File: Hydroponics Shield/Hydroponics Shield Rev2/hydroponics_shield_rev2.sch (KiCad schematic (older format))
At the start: 85 parts, among them CON1 PJ-202A, J1 282836-6, J2 282836-6, J3 RJHSE-5080, P2 0022053031, P3 MTG, P4 22-05-3021, P5 22-05-3021, P6 MTG, P7 MTG, P8 MTG, P9 0731000105, Q1 DMN65D8L-7, Q5 PSMN022-30PL,127, Q6 PSMN022-30PL,127, Q7 PSMN022-30PL,127, Q8 PSMN022-30PL,127, Q9 PSMN022-30PL,127, U1 LMC6482IN, U2 PCF8563, U3 AZ1117CH-3_3TRG1, Y1 CFS-20632768DZFB

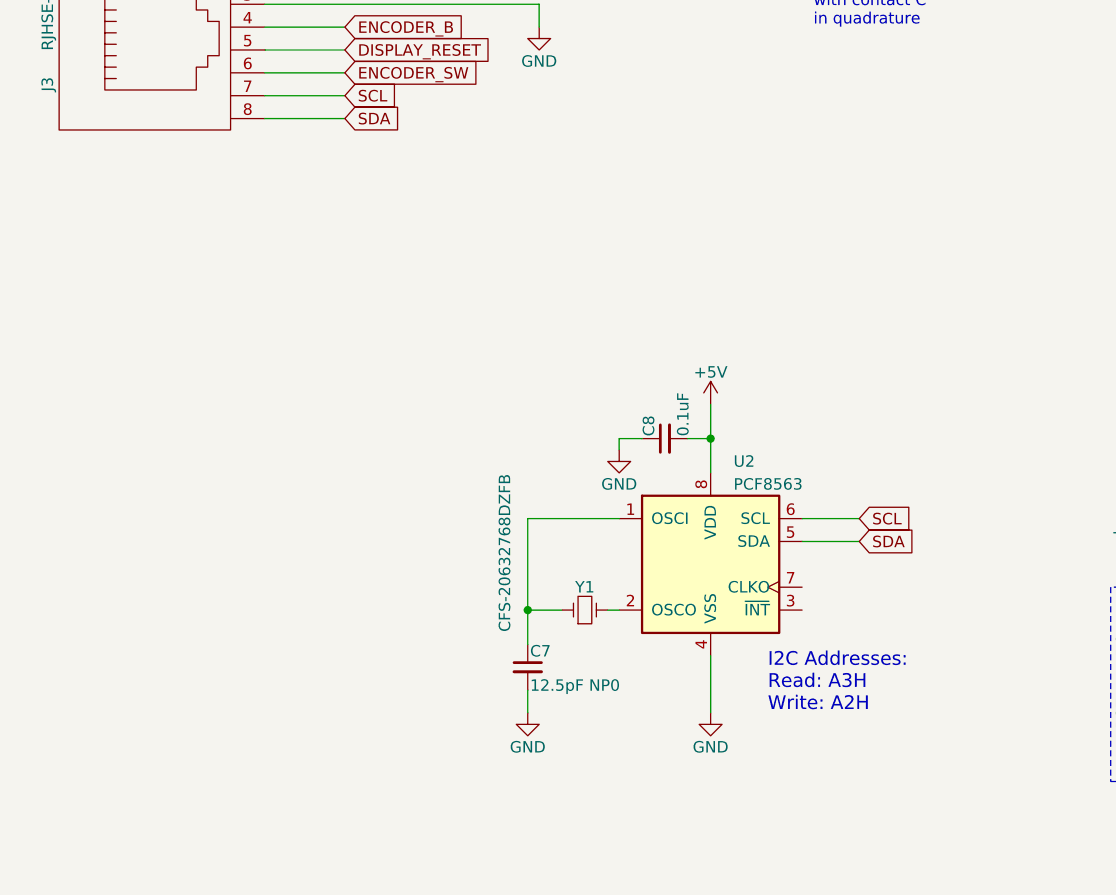
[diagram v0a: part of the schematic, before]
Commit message: .
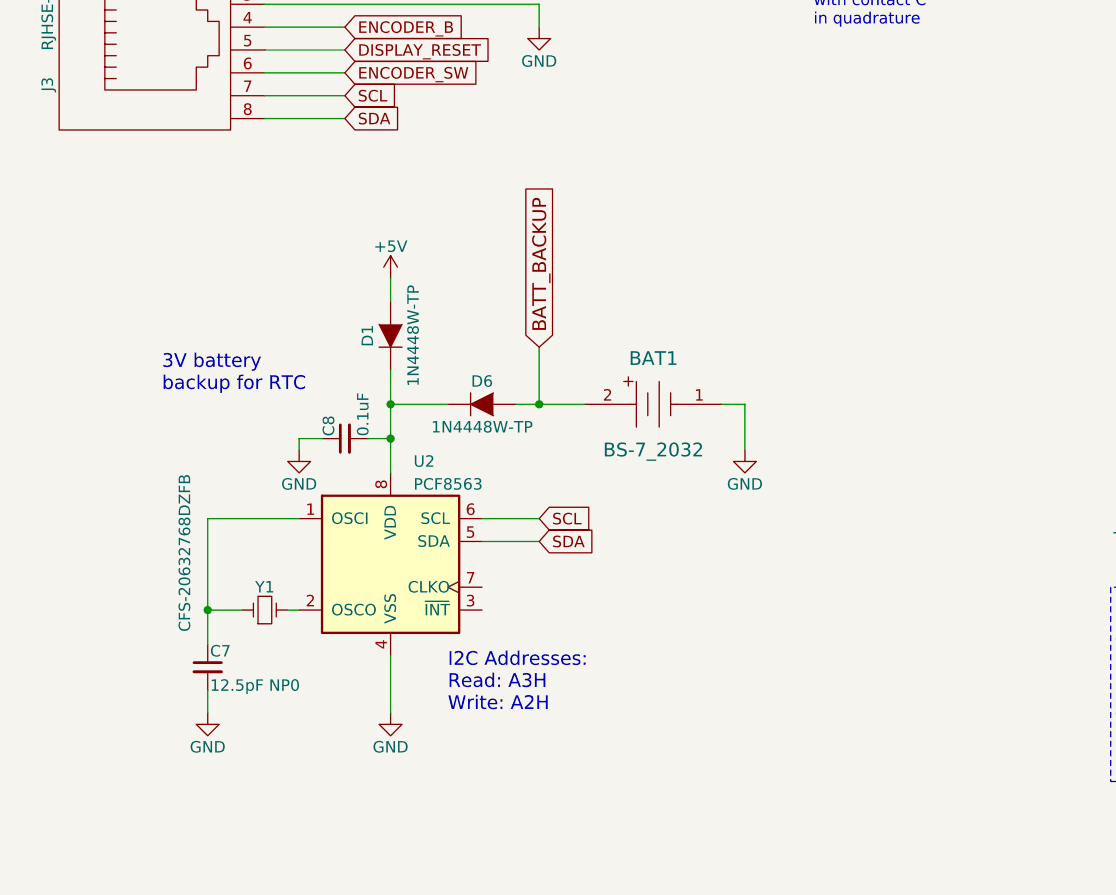
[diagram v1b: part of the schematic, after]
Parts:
- added BAT1: BS-7_2032, USER_CONNECTORS:BS-7_USER, symbol BS-7_2032
- added D1, D6: 1N4448W-TP, Diodes_SMD:SOD-123, symbol 1N4448W-TP
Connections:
- net +5V: now also D1.2 (A); no longer C8.2, U2.8 (VDD)
- net GND: now also BAT1.1
- new net: C8.2, D1.1 (K), D6.1 (K), U2.8 (VDD)
- new net BATT_BACKUP: BAT1.2, D6.2 (A)
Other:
- note added: "3V battery \nbackup for RTC"
- moved on the sheet: C7, C8, U2, Y1
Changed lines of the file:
@@
 L PCF8563 U2
 U 1 1 5B08C32E
-P 3750 9100
-F 0 "U2" H 3850 9550 50  0000 L CNN
-F 1 "PCF8563" H 3850 9450 50  0000 L CNN
-F 2 "digikey-footprints:8-SOIC" H 3750 9100 50  0001 C CNN
-F 3 "" H 3750 9100 50  0000 C CNN
-	1    3750 9100
-	1    0    0    -1
-$EndComp
-Wire Wire Line
-	3350 8900 2950 8900
-Wire Wire Line
-	2950 8900 2950 9450
-Wire Wire Line
-	2950 9300 3100 9300
-Wire Wire Line
-	3300 9300 3350 9300
-Connection ~ 2950 9300
+P 2350 9100
+F 0 "U2" H 2450 9550 50  0000 L CNN
+F 1 "PCF8563" H 2450 9450 50  0000 L CNN
+F 2 "digikey-footprints:8-SOIC" H 2350 9100 50  0001 C CNN
+F 3 "" H 2350 9100 50  0000 C CNN
+	1    2350 9100
+	1    0    0    -1
+$EndComp
+Wire Wire Line
+	1950 8900 1550 8900
+Wire Wire Line
+	1550 8900 1550 9450
+Wire Wire Line
+	1550 9300 1700 9300
+Wire Wire Line
+	1900 9300 1950 9300
+Connection ~ 1550 9300
 $Comp
 L C_Small C7
 U 1 1 5B091E53
-P 2950 9550
-F 0 "C7" H 2960 9620 50  0000 L CNN
-F 1 "12.5pF NP0" H 2960 9470 50  0000 L CNN
-F 2 "Capacitors_SMD:C_0805_HandSoldering" H 2950 9550 50  0001 C CNN
-F 3 "" H 2950 9550 50  0000 C CNN
-	1    2950 9550
-	1    0    0    -1
-$EndComp
-Wire Wire Line
-	2950 9650 2950 9750
+P 1550 9550
+F 0 "C7" H 1560 9620 50  0000 L CNN
+F 1 "12.5pF NP0" H 1560 9470 50  0000 L CNN
+F 2 "Capacitors_SMD:C_0805_HandSoldering" H 1550 9550 50  0001 C CNN
+F 3 "" H 1550 9550 50  0000 C CNN
+	1    1550 9550
+	1    0    0    -1
+$EndComp
+Wire Wire Line
+	1550 9650 1550 9750
 $Comp
 L GND #PWR051
 U 1 1 5B09286D
-P 2950 9750
-F 0 "#PWR051" H 2950 9500 50  0001 C CNN
-F 1 "GND" H 2950 9600 50  0000 C CNN
-F 2 "" H 2950 9750 50  0000 C CNN
-F 3 "" H 2950 9750 50  0000 C CNN
-	1    2950 9750
+P 1550 9750
+F 0 "#PWR051" H 1550 9500 50  0001 C CNN
+F 1 "GND" H 1550 9600 50  0000 C CNN
+F 2 "" H 1550 9750 50  0000 C CNN
+F 3 "" H 1550 9750 50  0000 C CNN
+	1    1550 9750
 	1    0    0    -1
 $EndComp
@@
 L GND #PWR052
 U 1 1 5B093393
-P 3750 9750
-F 0 "#PWR052" H 3750 9500 50  0001 C CNN
-F 1 "GND" H 3750 9600 50  0000 C CNN
-F 2 "" H 3750 9750 50  0000 C CNN
-F 3 "" H 3750 9750 50  0000 C CNN
-	1    3750 9750
-	1    0    0    -1
-$EndComp
-Wire Wire Line
-	3750 9500 3750 9750
-Wire Wire Line
-	3750 8400 3750 8700
+P 2350 9750
+F 0 "#PWR052" H 2350 9500 50  0001 C CNN
+F 1 "GND" H 2350 9600 50  0000 C CNN
+F 2 "" H 2350 9750 50  0000 C CNN
+F 3 "" H 2350 9750 50  0000 C CNN
+	1    2350 9750
+	1    0    0    -1
+$EndComp
+Wire Wire Line
+	2350 9500 2350 9750
+Wire Wire Line
+	2350 8250 2350 8700
 $Comp
 L +5V #PWR053
 U 1 1 5B0942AC
-P 3750 8400
-F 0 "#PWR053" H 3750 8250 50  0001 C CNN
-F 1 "+5V" H 3750 8540 50  0000 C CNN
-F 2 "" H 3750 8400 50  0000 C CNN
-F 3 "" H 3750 8400 50  0000 C CNN
-	1    3750 8400
+P 2350 7850
+F 0 "#PWR053" H 2350 7700 50  0001 C CNN
+F 1 "+5V" H 2350 7990 50  0000 C CNN
+F 2 "" H 2350 7850 50  0000 C CNN
+F 3 "" H 2350 7850 50  0000 C CNN
+	1    2350 7850
 	-1   0    0    -1
 $EndComp
@@
 L C_Small C8
 U 1 1 5B094D20
-P 3550 8550
-F 0 "C8" H 3560 8620 50  0000 L CNN
-F 1 "0.1uF" H 3560 8470 50  0000 L CNN
-F 2 "Capacitors_SMD:C_0805_HandSoldering" H 3550 8550 50  0001 C CNN
-F 3 "" H 3550 8550 50  0000 C CNN
-	1    3550 8550
+P 2150 8550
+F 0 "C8" H 2160 8620 50  0000 L CNN
+F 1 "0.1uF" H 2160 8470 50  0000 L CNN
+F 2 "Capacitors_SMD:C_0805_HandSoldering" H 2150 8550 50  0001 C CNN
+F 3 "" H 2150 8550 50  0000 C CNN
+	1    2150 8550
 	0    -1   -1   0
 $EndComp
 Wire Wire Line
-	3750 8550 3650 8550
-Connection ~ 3750 8550
+	2350 8550 2250 8550
+Connection ~ 2350 8550
 $Comp
 L GND #PWR054
 U 1 1 5B0957DA
-P 3350 8600
-F 0 "#PWR054" H 3350 8350 50  0001 C CNN
-F 1 "GND" H 3350 8450 50  0000 C CNN
-F 2 "" H 3350 8600 50  0000 C CNN
-F 3 "" H 3350 8600 50  0000 C CNN
-	1    3350 8600
-	1    0    0    -1
-$EndComp
-Wire Wire Line
-	3450 8550 3350 8550
-Wire Wire Line
-	3350 8550 3350 8600
+P 1950 8600
+F 0 "#PWR054" H 1950 8350 50  0001 C CNN
+F 1 "GND" H 1950 8450 50  0000 C CNN
+F 2 "" H 1950 8600 50  0000 C CNN
+F 3 "" H 1950 8600 50  0000 C CNN
+	1    1950 8600
+	1    0    0    -1
+$EndComp
+Wire Wire Line
+	2050 8550 1950 8550
+Wire Wire Line
+	1950 8550 1950 8600
 $Comp
 L R R4
@@
 Text Notes 8600 10450 0    60   ~ 0
 TODO:\nverify I2C addresses will not conflict
-Text Notes 4000 9750 0    60   ~ 0
+Text Notes 2600 9750 0    60   ~ 0
 I2C Addresses:\nRead: A3H\nWrite: A2H\n
-Text GLabel 4400 9000 2    50   Input ~ 0
+Text GLabel 3000 9000 2    50   Input ~ 0
 SDA
-Text GLabel 4400 8900 2    50   Input ~ 0
+Text GLabel 3000 8900 2    50   Input ~ 0
 SCL
 Wire Wire Line
-	4400 8900 4150 8900
-Wire Wire Line
-	4400 9000 4150 9000
+	3000 8900 2750 8900
+Wire Wire Line
+	3000 9000 2750 9000
 Text GLabel 2150 7150 2    50   Input ~ 0
 SDA
@@
 L CFS-20632768DZFB Y1
 U 1 1 5B0DF230
-P 3200 9300
-F 0 "Y1" H 3200 9400 50  0000 C CNN
-F 1 "CFS-20632768DZFB" V 2850 9550 50  0000 C CNN
-F 2 "Crystals:Crystal_Round_Horizontal_2mm" H 3100 9300 50  0001 C CNN
-F 3 "" H 3200 9300 50  0000 C CNN
-	1    3200 9300
+P 1800 9300
+F 0 "Y1" H 1800 9400 50  0000 C CNN
+F 1 "CFS-20632768DZFB" V 1450 9550 50  0000 C CNN
+F 2 "Crystals:Crystal_Round_Horizontal_2mm" H 1700 9300 50  0001 C CNN
+F 3 "" H 1800 9300 50  0000 C CNN
+	1    1800 9300
 	1    0    0    -1
 $EndComp
@@
 Text Notes 8300 5400 0    60   ~ 0
 offset zero jumper
+Text Notes 1350 8350 0    60   ~ 0
+3V battery \nbackup for RTC
+Wire Wire Line
+	2900 8400 3200 8400
+Wire Wire Line
+	2600 8400 2350 8400
+Connection ~ 2350 8400
+Wire Wire Line
+	3800 8400 3900 8400
+Wire Wire Line
+	3900 8400 3900 8600
+$Comp
+L GND #PWR062
+U 1 1 5B24017F
+P 3900 8600
+F 0 "#PWR062" H 3900 8350 50  0001 C CNN
+F 1 "GND" H 3900 8450 50  0000 C CNN
+F 2 "" H 3900 8600 50  0000 C CNN
+F 3 "" H 3900 8600 50  0000 C CNN
+	1    3900 8600
+	1    0    0    -1
+$EndComp
+$Comp
+L 1N4448W-TP D1
+U 1 1 5B24135C
+P 2350 8100
+F 0 "D1" H 2350 8200 50  0000 C CNN
+F 1 "1N4448W-TP" H 2350 8000 50  0000 C CNN
+F 2 "Diodes_SMD:SOD-123" H 2250 8100 50  0001 C CNN
+F 3 "" H 2350 8100 50  0000 C CNN
+	1    2350 8100
+	0    -1   -1   0
+$EndComp
+Wire Wire Line
+	2350 7850 2350 7950
+$Comp
+L 1N4448W-TP D6
+U 1 1 5B241DC4
+P 2750 8400
+F 0 "D6" H 2750 8500 50  0000 C CNN
+F 1 "1N4448W-TP" H 2750 8300 50  0000 C CNN
+F 2 "Diodes_SMD:SOD-123" H 2650 8400 50  0001 C CNN
+F 3 "" H 2750 8400 50  0000 C CNN
+	1    2750 8400
+	1    0    0    -1
+$EndComp
+Wire Wire Line
+	3000 8400 3000 8150
+Connection ~ 3000 8400
+Text GLabel 3000 8150 1    60   Input ~ 0
+BATT_BACKUP
+$Comp
+L BS-7_2032 BAT1
+U 1 1 5B24898A
+P 3500 8400
+F 0 "BAT1" H 3500 8600 60  0000 C CNN
+F 1 "BS-7_2032" H 3500 8200 60  0000 C CNN
+F 2 "USER_CONNECTORS:BS-7_USER" H 3700 8600 60  0001 L CNN
+F 3 "http://www.memoryprotectiondevices.com/datasheets/BS-7-datasheet.pdf" H 3700 8700 60  0001 L CNN
+F 4 "BS-7-ND" H 3700 8800 60  0001 L CNN "Digi-Key_PN"
+F 5 "BS-7" H 3700 8900 60  0001 L CNN "MPN"
+F 6 "Battery Products" H 3700 9000 60  0001 L CNN "Category"
+F 7 "Battery Holders, Clips, Contacts" H 3700 9100 60  0001 L CNN "Family"
+F 8 "http://www.memoryprotectiondevices.com/datasheets/BS-7-datasheet.pdf" H 3700 9200 60  0001 L CNN "DK_Datasheet_Link"
+F 9 "/product-detail/en/mpd-memory-protection-devices/BS-7/BS-7-ND/389447" H 3700 9300 60  0001 L CNN "DK_Detail_Page"
+F 10 "HOLDER COINCELL 2032 RETAINRCLIP" H 3700 9400 60  0001 L CNN "Description"
+F 11 "MPD (Memory Protection Devices)" H 3700 9500 60  0001 L CNN "Manufacturer"
+	1    3500 8400
+	1    0    0    -1
+$EndComp
 $EndSCHEMATC
